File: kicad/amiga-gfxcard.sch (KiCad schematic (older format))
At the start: 29 parts, among them P1 ADDR1, P2 ADDR2, P3 ADDR3, P4 DATA1, P5 DATA2, P6 CTRL_IN, P7 CTRL_OUT, U1 74LVC8T245, U2 74LVC8T245, U3 74LVC8T245, U4 74LVC8T245, U5 74LVC8T245, U6 74LVC8T245

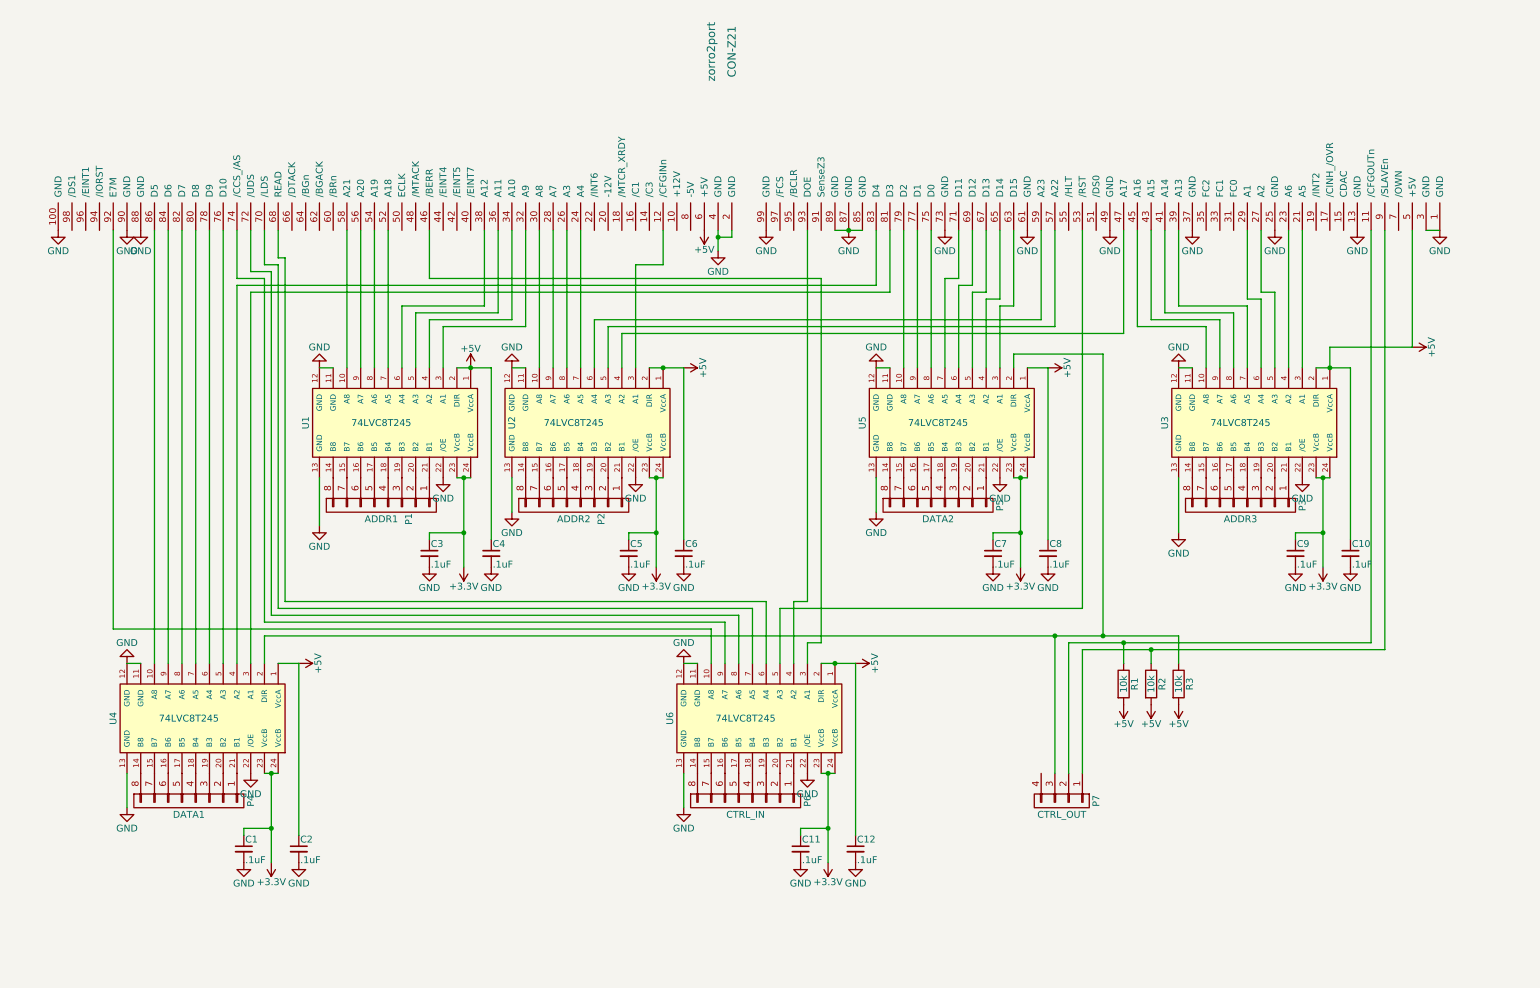
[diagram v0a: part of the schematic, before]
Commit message: redo of mk2 board finished
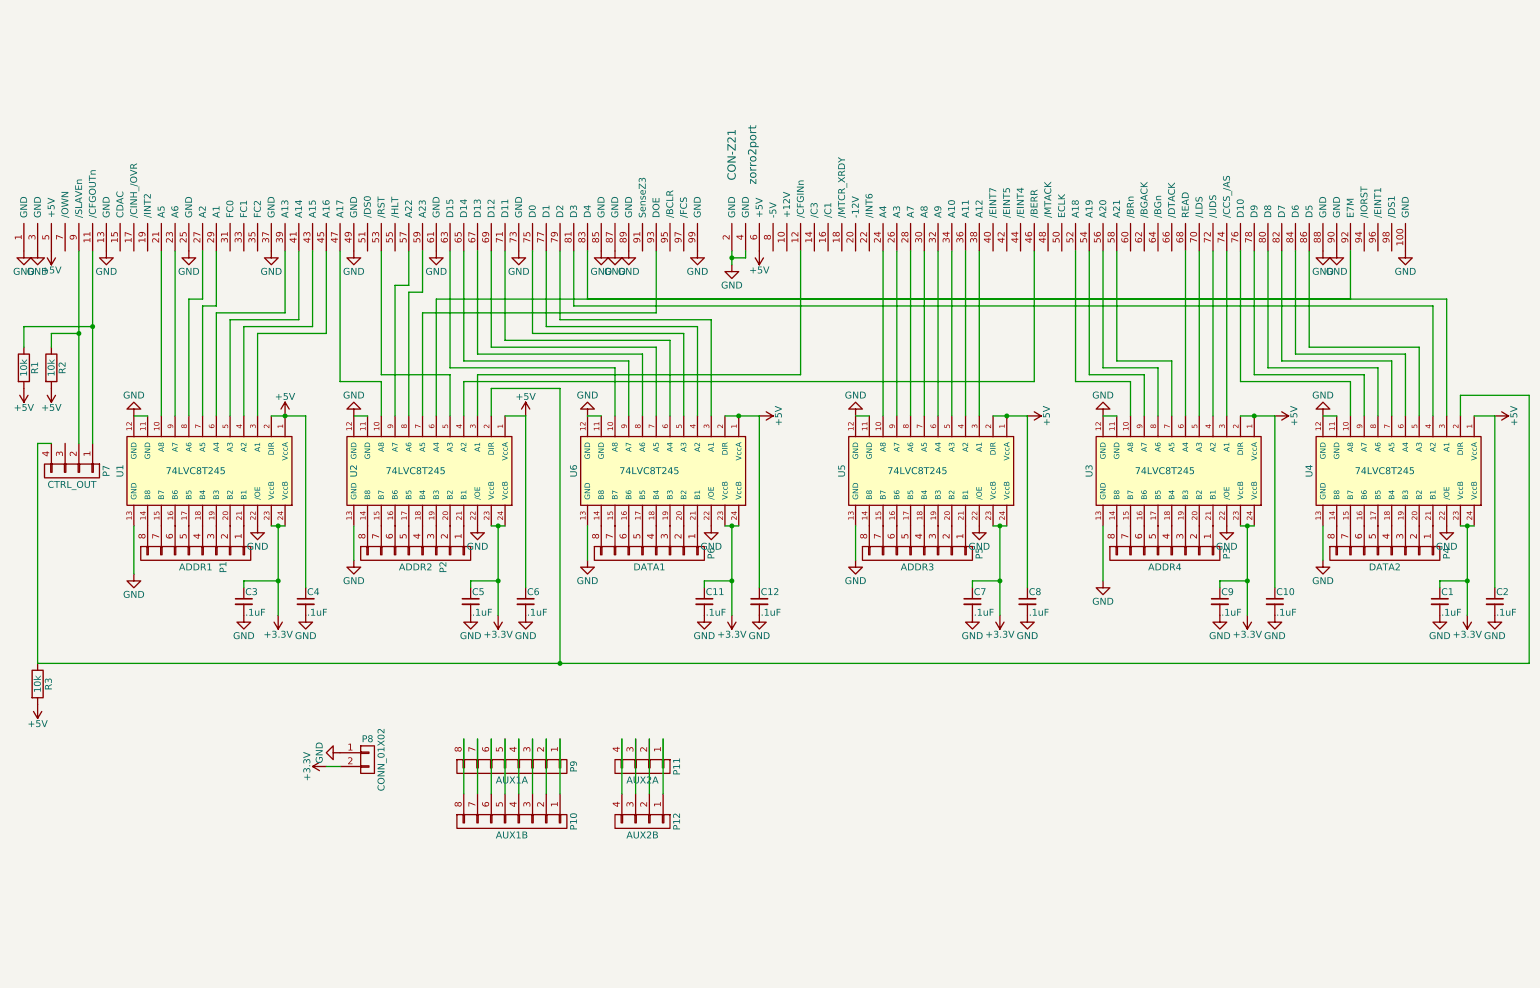
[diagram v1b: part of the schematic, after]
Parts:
- added P10: AUX1B, Pin_Headers:Pin_Header_Straight_1x08, symbol CONN_01X08
- added P11: AUX2A, Pin_Headers:Pin_Header_Straight_1x04, symbol CONN_01X04
- added P12: AUX2B, Pin_Headers:Pin_Header_Straight_1x04, symbol CONN_01X04
- added P8: CONN_01X02, Pin_Headers:Pin_Header_Straight_1x02, symbol CONN_01X02
- added P9: AUX1A, Pin_Headers:Pin_Header_Straight_1x08, symbol CONN_01X08
- C1, C10, C11, C12, C2, C3, C4, C5, C6, C7, C8, C9: footprint Capacitors_ThroughHole:C_Rect_L4_W2.5_P2.5 -> Capacitors_SMD:C_0805_HandSoldering
- P3: value ADDR3 -> ADDR4
- P4: value DATA1 -> DATA2
- P5: value DATA2 -> ADDR3
- P6: value CTRL_IN -> DATA1
- R1, R2, R3: footprint Resistors_ThroughHole:Resistor_Horizontal_RM7mm -> Resistors_SMD:R_1206_HandSoldering
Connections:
- net +3V3: now also P8.2 (P2)
- net +5V: now also U5.2 (DIR); no longer U2.2 (DIR)
- net GND: now also P8.1 (P1)
- net at CON-Z21.11 (/CFGOUTn), R1.1: now also P7.1 (P1); no longer P7.2 (P2)
- net at CON-Z21.21 (A5): now also U1.10 (A8); no longer U3.3 (A1)
- net at CON-Z21.23 (A6): now also U1.9 (A7); no longer U3.4 (A2)
- net at CON-Z21.24 (A4): now also U5.10 (A8); no longer U2.7 (A5)
- net at CON-Z21.26 (A3): now also U5.9 (A7); no longer U2.8 (A6)
- net at CON-Z21.27 (A2): now also U1.8 (A6); no longer U3.5 (A3)
- net at CON-Z21.28 (A7): now also U5.8 (A6); no longer U2.9 (A7)
- net at CON-Z21.29 (A1): now also U1.7 (A5); no longer U3.6 (A4)
- net at CON-Z21.30 (A8): now also U5.7 (A5); no longer U2.10 (A8)
- net at CON-Z21.32 (A9): now also U5.6 (A4); no longer U1.3 (A1)
- net at CON-Z21.34 (A10): now also U5.5 (A3); no longer U1.4 (A2)
- net at CON-Z21.36 (A11): now also U5.4 (A2); no longer U1.5 (A3)
- net at CON-Z21.38 (A12): now also U5.3 (A1); no longer U1.6 (A4)
- net at CON-Z21.39 (A13): now also U1.6 (A4); no longer U3.7 (A5)
- net at CON-Z21.41 (A14): now also U1.5 (A3); no longer U3.8 (A6)
- net at CON-Z21.43 (A15): now also U1.4 (A2); no longer U3.9 (A7)
- net at CON-Z21.45 (A16): now also U1.3 (A1); no longer U3.10 (A8)
- net at CON-Z21.46 (/BERR): now also U2.4 (A2); no longer U6.3 (A1)
- net at CON-Z21.47 (A17): now also U2.10 (A8); no longer U2.4 (A2)
- net at CON-Z21.52 (A18): now also U3.10 (A8); no longer U1.7 (A5)
- net at CON-Z21.53 (/RST): now also U2.5 (A3); no longer U6.5 (A3)
- net at CON-Z21.54 (A19): now also U3.9 (A7); no longer U1.8 (A6)
- net at CON-Z21.56 (A20): now also U3.8 (A6); no longer U1.9 (A7)
- net at CON-Z21.57 (A22): now also U2.9 (A7); no longer U2.5 (A3)
- net at CON-Z21.58 (A21): now also U3.7 (A5); no longer U1.10 (A8)
- net at CON-Z21.59 (A23): now also U2.8 (A6); no longer U2.6 (A4)
- net at CON-Z21.63 (D15): now also U6.10 (A8); no longer U5.3 (A1)
- net at CON-Z21.65 (D14): now also U6.9 (A7); no longer U5.4 (A2)
- net at CON-Z21.67 (D13): now also U6.8 (A6); no longer U5.5 (A3)
- net at CON-Z21.68 (READ): now also U3.6 (A4); no longer U6.6 (A4)
- net at CON-Z21.69 (D12): now also U6.7 (A5); no longer U5.6 (A4)
- net at CON-Z21.70 (/LDS): now also U3.5 (A3); no longer U6.7 (A5)
- net at CON-Z21.71 (D11): now also U6.6 (A4); no longer U5.7 (A5)
- net at CON-Z21.72 (/UDS): now also U3.4 (A2); no longer U6.8 (A6)
- net at CON-Z21.74 (/CCS_/AS): now also U3.3 (A1); no longer U6.9 (A7)
- net at CON-Z21.75 (D0): now also U6.5 (A3); no longer U5.8 (A6)
- net at CON-Z21.76 (D10): now also U4.10 (A8); no longer U4.5 (A3)
- net at CON-Z21.77 (D1): now also U6.4 (A2); no longer U5.9 (A7)
- net at CON-Z21.78 (D9): now also U4.9 (A7); no longer U4.6 (A4)
- net at CON-Z21.79 (D2): now also U6.3 (A1); no longer U5.10 (A8)
- net at CON-Z21.80 (D8): now also U4.8 (A6); no longer U4.7 (A5)
- net at CON-Z21.81 (D3): now also U4.4 (A2); no longer U4.3 (A1)
- net at CON-Z21.82 (D7): now also U4.7 (A5); no longer U4.8 (A6)
- net at CON-Z21.83 (D4): now also CON-Z21.92 (E7M), U2.6 (A4), U4.3 (A1); no longer U4.4 (A2)
- net at CON-Z21.84 (D6): now also U4.6 (A4); no longer U4.9 (A7)
- net at CON-Z21.86 (D5): now also U4.5 (A3); no longer U4.10 (A8)
- net at CON-Z21.9 (/SLAVEn), R2.1: now also P7.2 (P2); no longer P7.1 (P1)
- net at CON-Z21.93 (DOE): now also U2.7 (A5); no longer U6.4 (A2)
- net at R3.1, U4.2 (DIR): now also P7.4 (P4), U2.2 (DIR); no longer P7.3 (P3), U5.2 (DIR)
- new net: P10.1 (P1), P9.1 (P1)
- new net: P10.2 (P2), P9.2 (P2)
- new net: P10.3 (P3), P9.3 (P3)
- new net: P10.4 (P4), P9.4 (P4)
- new net: P10.5 (P5), P9.5 (P5)
- new net: P10.6 (P6), P9.6 (P6)
- new net: P10.7 (P7), P9.7 (P7)
- new net: P10.8 (P8), P9.8 (P8)
- new net: P11.1 (P1), P12.1 (P1)
- new net: P11.2 (P2), P12.2 (P2)
- new net: P11.3 (P3), P12.3 (P3)
- new net: P11.4 (P4), P12.4 (P4)
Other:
- moved on the sheet: C1, C10, C11, C12, C2, C3, C4, C5, C6, C7, C8, C9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
